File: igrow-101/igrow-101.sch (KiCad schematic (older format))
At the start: 26 parts, among them P1 CONN_02X05, Q1 NPN, Q2 NPN, Q3 NPN, SW1 SW_PUSH, U1 NRF51822-MODULE, U2 SHT21, U3 TL972

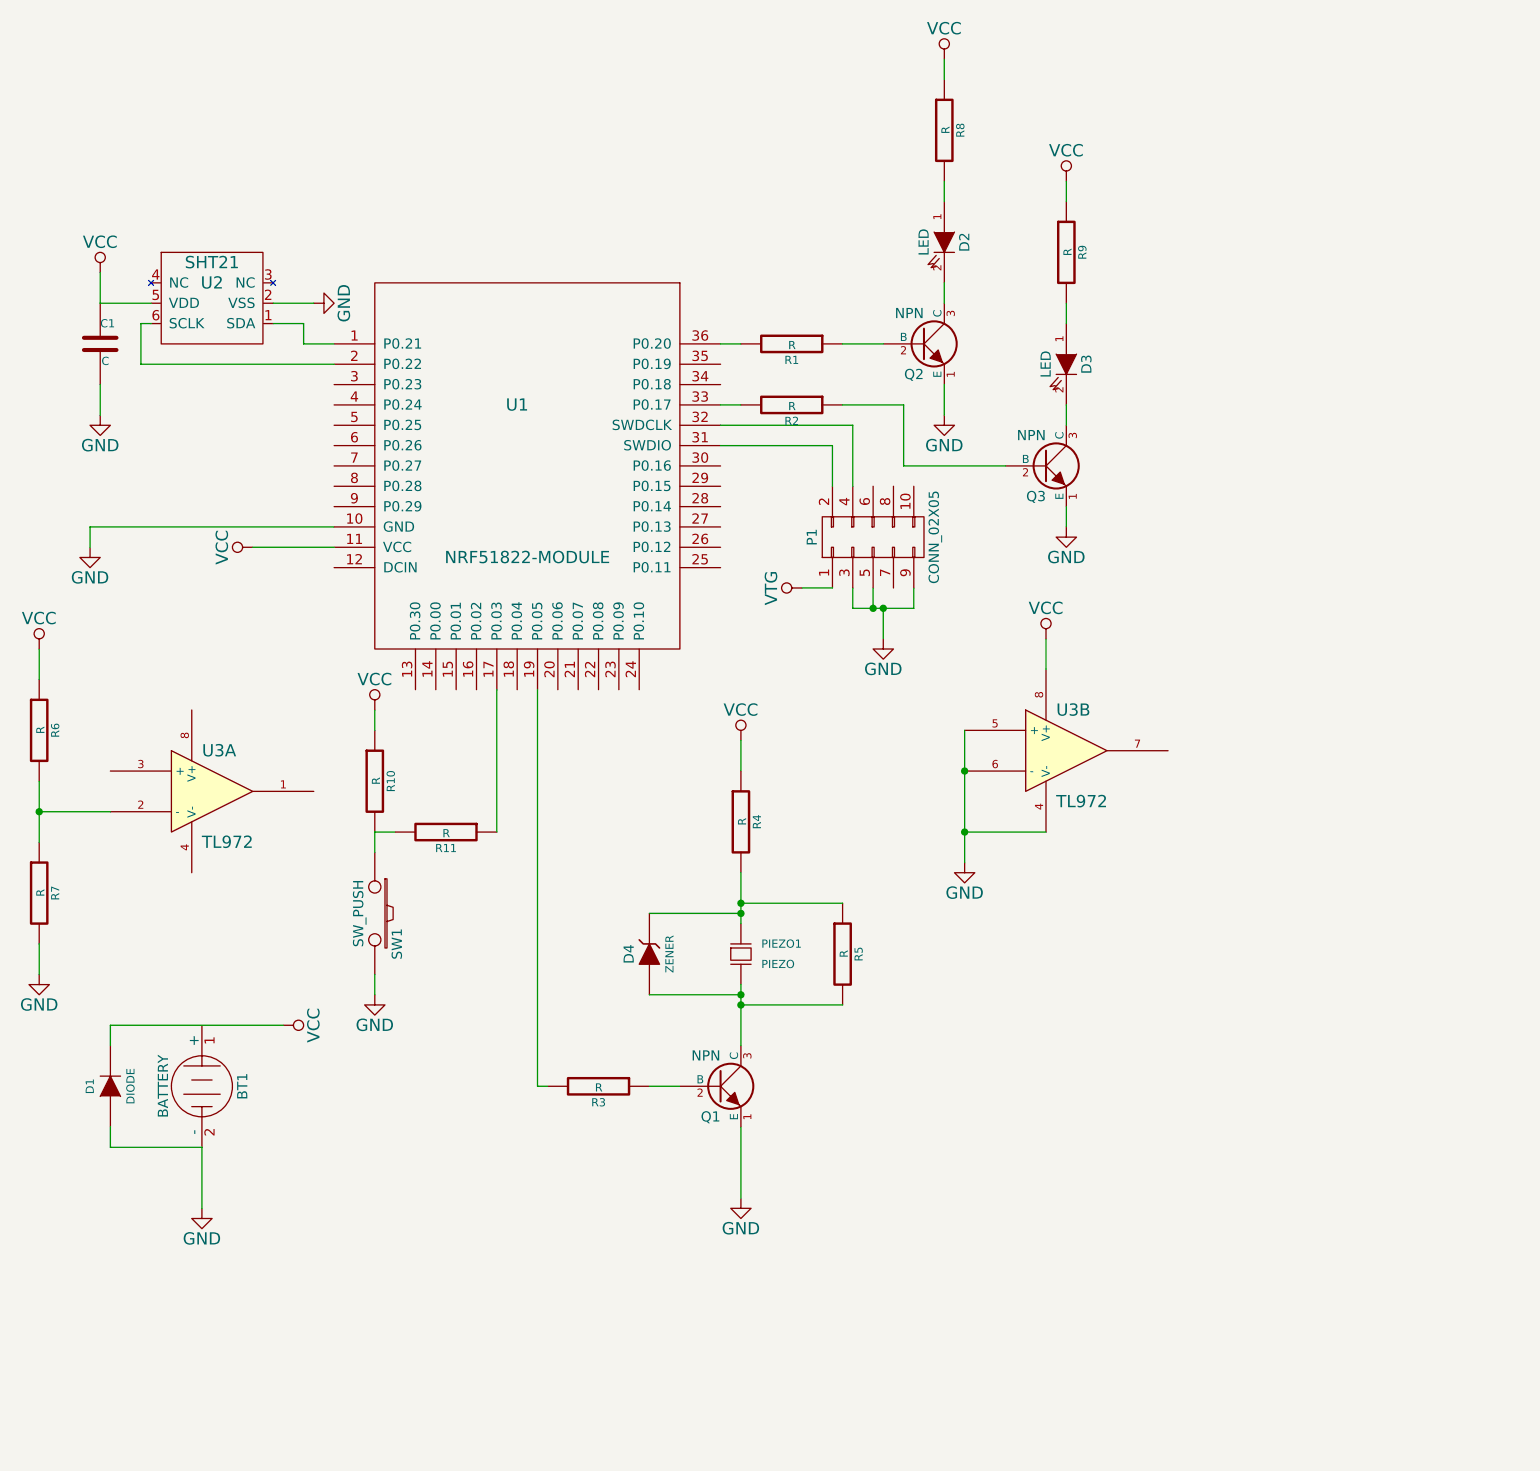
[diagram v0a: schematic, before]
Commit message: Post autorouting
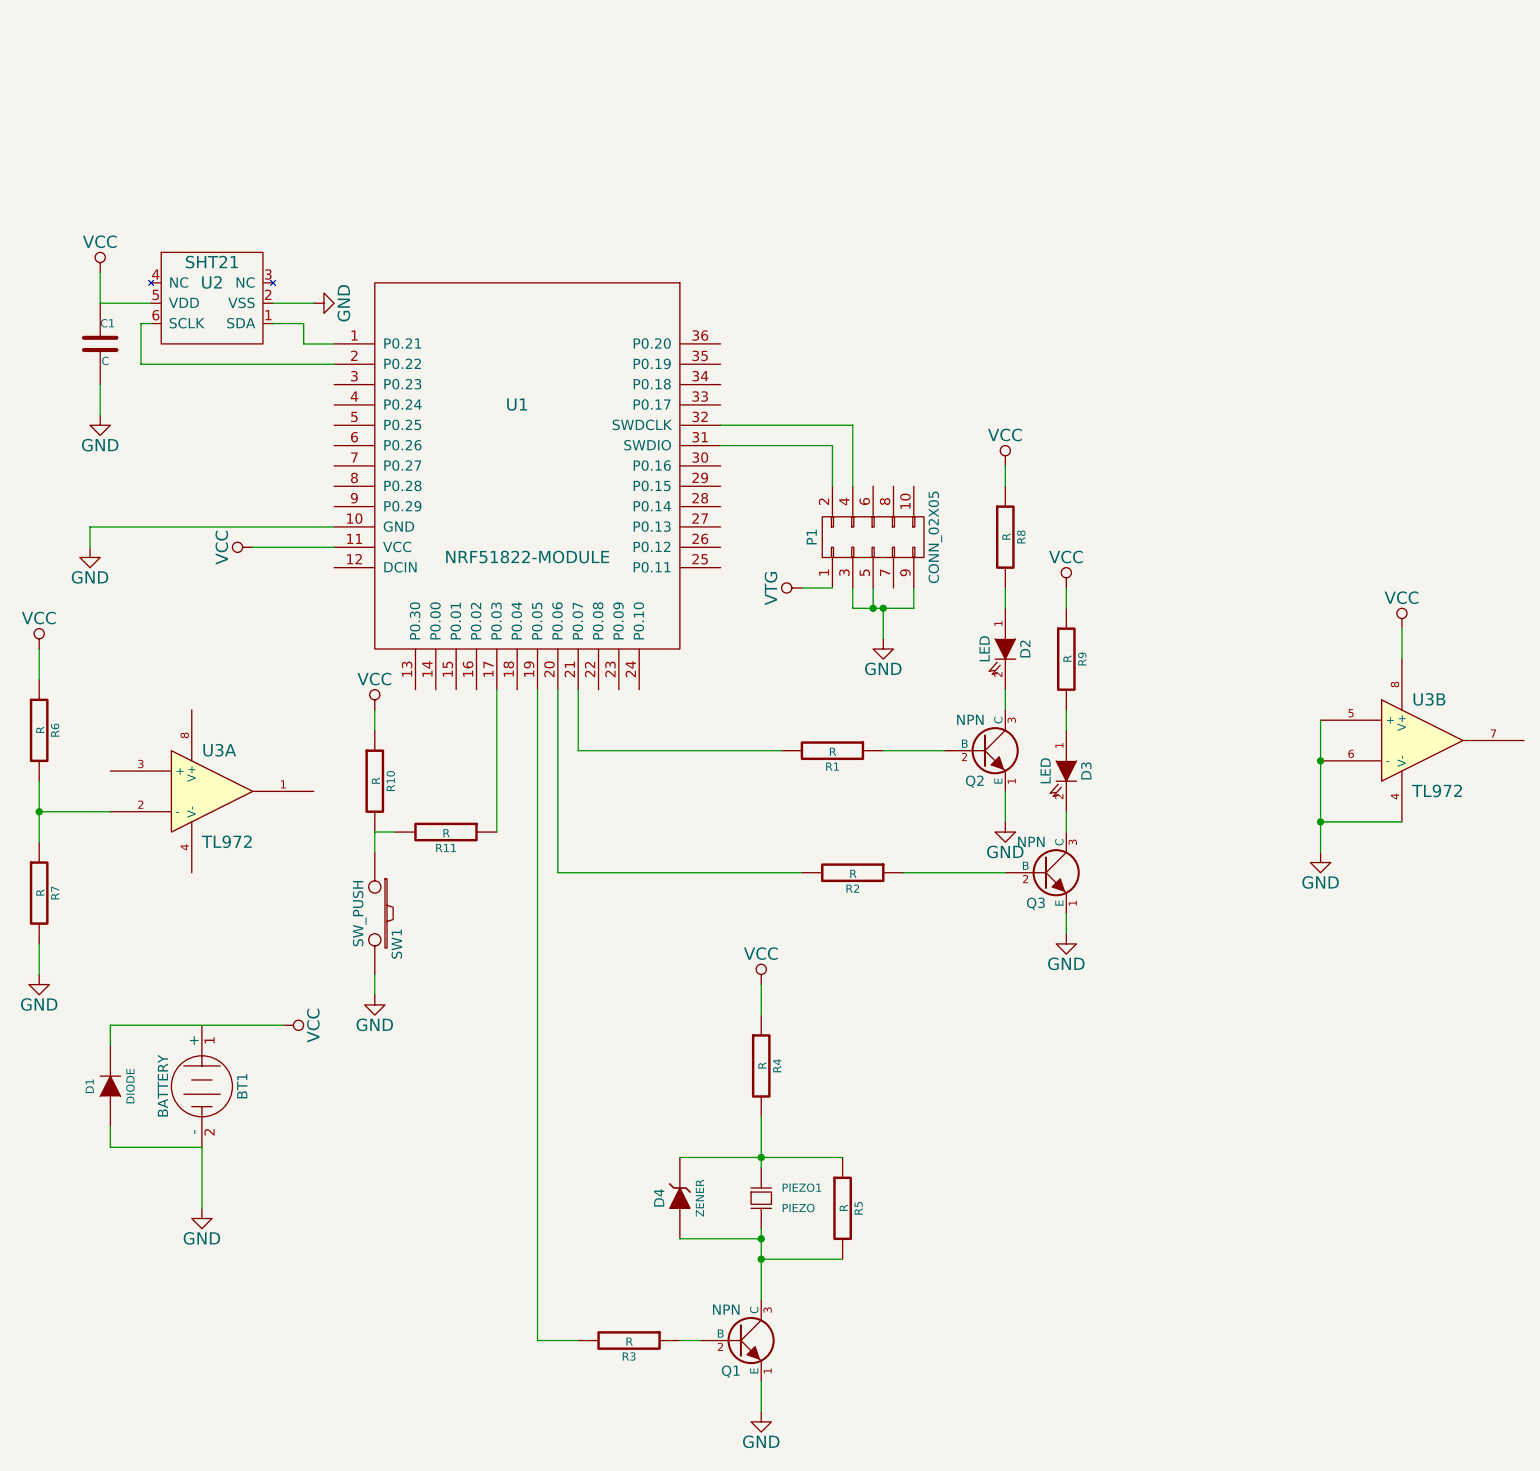
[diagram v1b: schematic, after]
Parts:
- BT1: footprint guan:BAT-BK912 -> igrow:CR2032_THRUHOLE
- PIEZO1: footprint Resistors_ThroughHole:Resistor_Horizontal_RM10mm -> Resistors_ThroughHole:Resistor_Vertical_RM5mm
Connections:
- net at U1.20 (P0.06): now also R2.2
- net at U1.21 (P0.07): now also R1.2
- net at U1.33 (P0.17): no longer R2.2
- net at U1.36 (P0.20): no longer R1.2
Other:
- moved on the sheet: D2, D3, D4, PIEZO1, Q1, Q2, Q3, R1, R2, R3, R4, R5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
